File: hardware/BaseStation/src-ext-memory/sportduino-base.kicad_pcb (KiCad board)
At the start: 2 copper layers, 76.8 x 45.7 mm, 42 parts, among them SW1 SW_Reed, X1 Battery, X2 Prog, X3 RC522

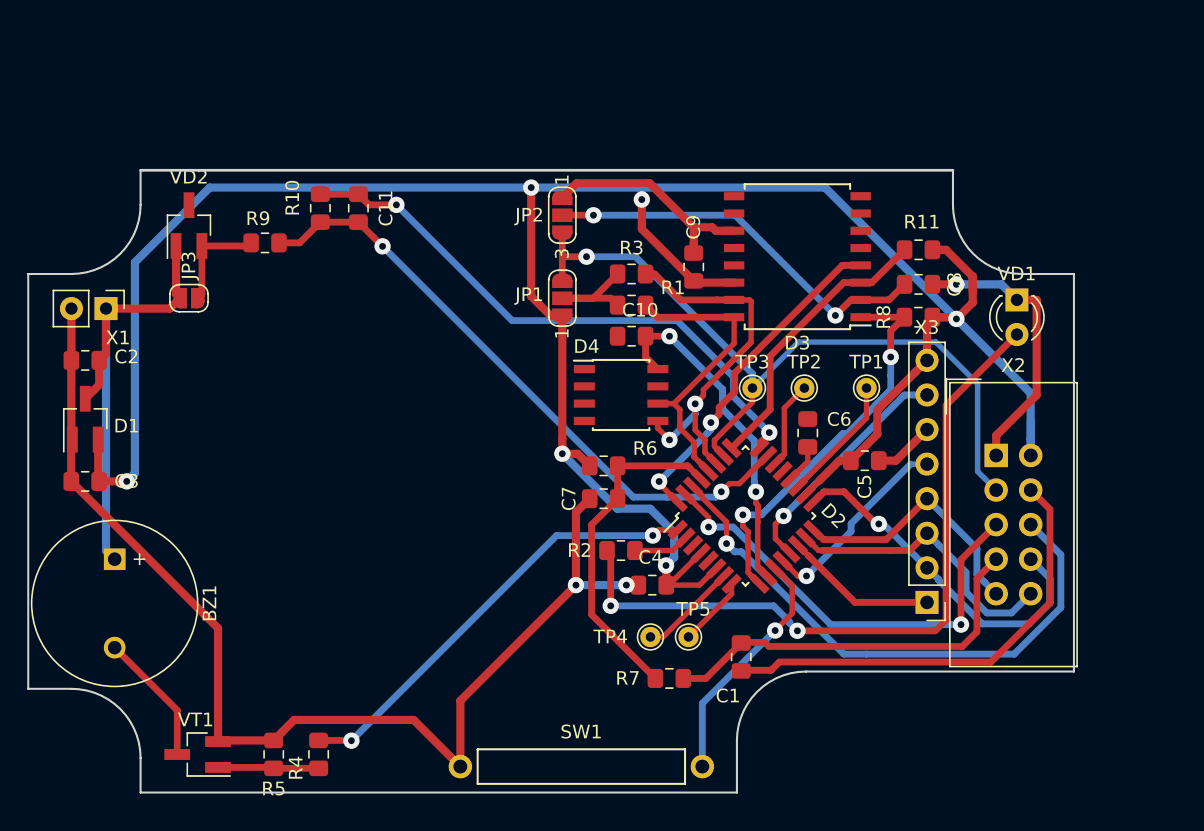
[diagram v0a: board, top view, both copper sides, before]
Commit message: Updated PCB
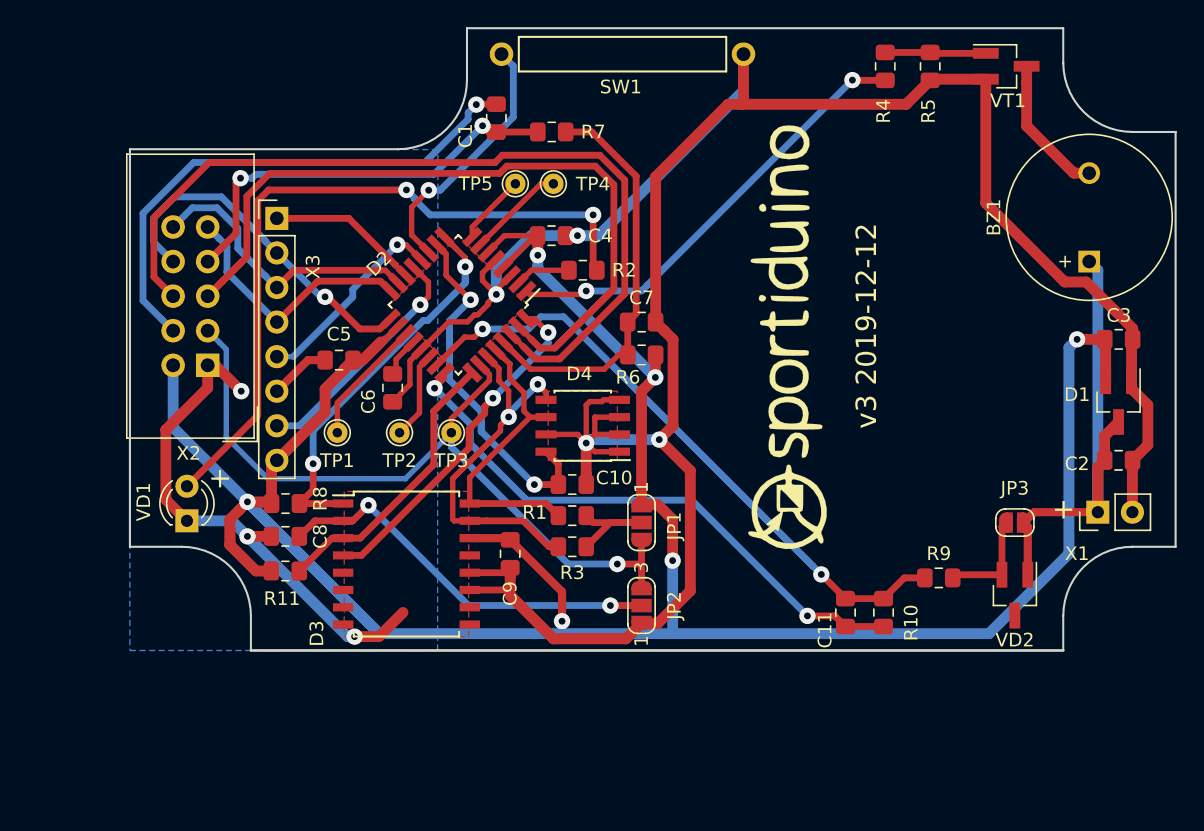
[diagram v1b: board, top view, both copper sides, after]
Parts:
- added G***: LOGO, src-ext-memory:logo, F.Cu at (182.1, 80.8)
- D3: value DS3231SN -> (none)
- moved VT1 78.0 mm to (198.2, 60.9), turned to 0 degrees
- moved C3 76.7 mm to (206.5, 81.0), turned to 0 degrees
- moved C2 76.3 mm to (206.5, 89.9), turned to 0 degrees
- moved D1 75.9 mm to (206.5, 85.6), turned to 270 degrees
- moved BZ1 74.9 mm to (204.3, 75.3), turned to 90 degrees
- moved X1 74.4 mm to (205.0, 93.7), turned to 90 degrees
- moved R5 69.9 mm to (192.6, 60.9), turned to 90 degrees
- moved VD2 66.5 mm to (198.9, 99.8), turned to 270 degrees
- moved R4 65.5 mm to (189.3, 60.9), turned to 270 degrees
- moved VD1 63.1 mm to (138.0, 94.3), turned to 90 degrees
- moved JP3 62.9 mm to (198.9, 94.5), turned to 180 degrees
- moved X2 58.3 mm to (139.6, 82.9), turned to 180 degrees
- moved X3 55.5 mm to (144.6, 72.1), turned to 0 degrees
- moved R9 55.3 mm to (193.3, 98.5), turned to 0 degrees
- moved SW1 52.4 mm to (170.0, 60.0), turned to 0 degrees
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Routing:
- net GNDD: track 126.1 -> 253.1 mm, vias 3 -> 7
- net TX: track 33.2 -> 69.9 mm, vias 2 -> 0
- net +3V3: track 190.1 -> 226.1 mm
- net RX: track 41.6 -> 63.1 mm, vias 1 -> 0
- net ADCIN: track 47.9 -> 69.2 mm
- net Net-(C7-Pad1): track 25.0 -> 32.7 mm
- net Net-(C1-Pad2): track 33.4 -> 39.1 mm, vias 0 -> 1
- net PD6: track 27.4 -> 31.9 mm
- net RST: track 28.9 -> 32.8 mm, vias 0 -> 2
- net 32K: track 31.0 -> 33.3 mm
- net Net-(D2-Pad11): track 17.8 -> 19.0 mm
- net Net-(BZ1-Pad2): track 9.75 -> 10.4 mm
- net Net-(D2-Pad32): track 25.2 -> 25.8 mm
- added copper zone on B.Cu, net GNDD
- added copper zone on F.Cu, net GNDD
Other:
- outline, holes or cut-outs redrawn
- net class power: trace_width 0.6 -> 0.8
- board text added: "+"
- board text added: "v3 2019-12-12"
